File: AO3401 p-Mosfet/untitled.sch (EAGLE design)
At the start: 5 parts

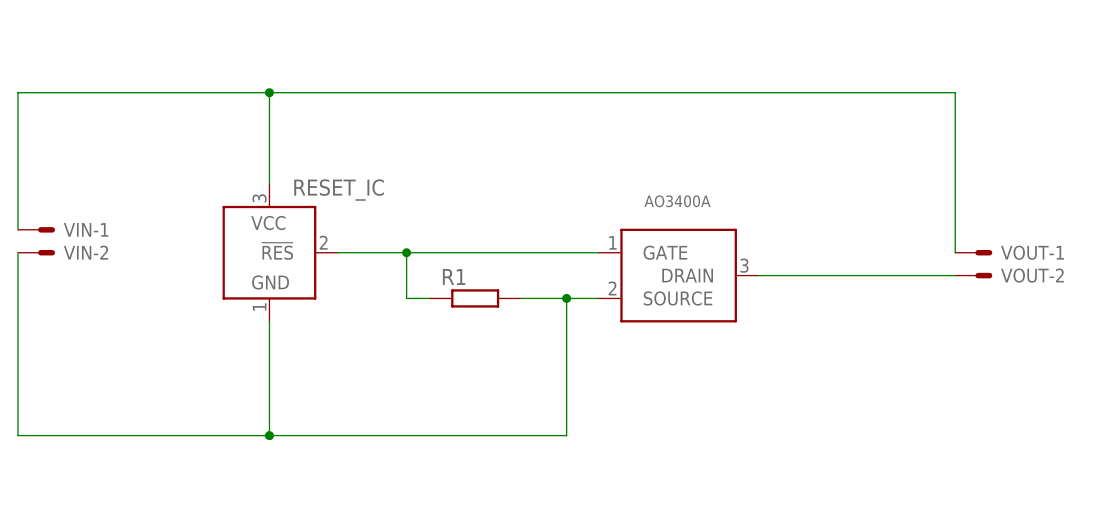
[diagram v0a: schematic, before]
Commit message: new update podlewacz v2
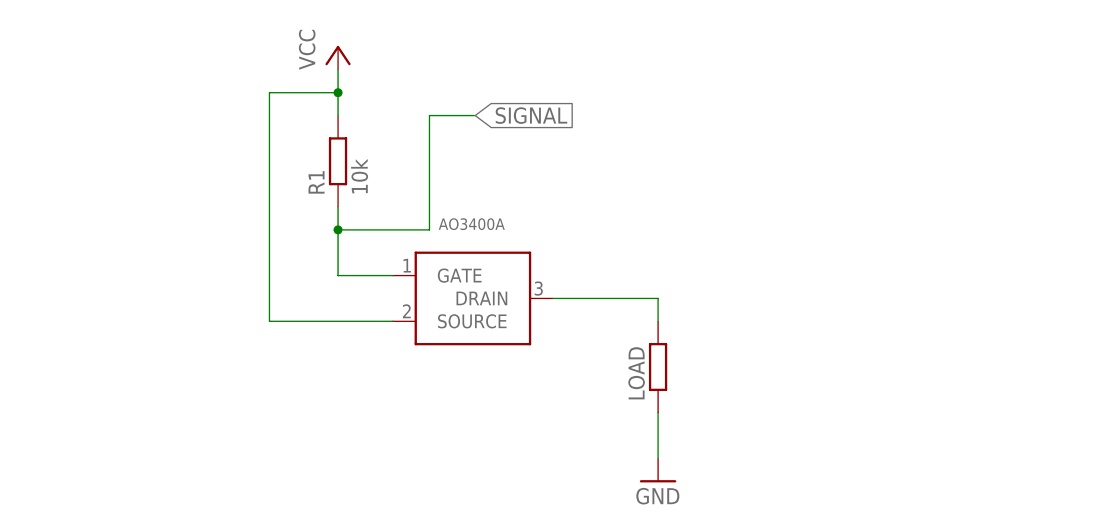
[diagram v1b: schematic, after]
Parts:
- removed MOSFET: AO3400A, smd-footprints:AO3400A
- removed RESET_IC: (no value), telcom:TCM809
- removed VIN, VOUT: 22-23-2021, con-molex:22-23-2021
- added AO3401_P-MOSFET: AO3401_P-MOSFET, smd-footprints:AO3400A
- added LOAD: (no value), resistor:R-EU_0204/2V
- R1: value (none) -> 10k; device resistor:R-EU_R1206 -> resistor:R-EU_0204/2V
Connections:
- removed net N$1: MOSFET.DRAIN, VOUT-2.S
- removed net N$3: MOSFET.GATE, R1.1, RESET_IC.!RES
- new net N$2: AO3401_P-MOSFET.DRAIN, LOAD.2
- new net SIGNAL: AO3401_P-MOSFET.GATE, R1.1
- net GND: now also LOAD.1; no longer MOSFET.SOURCE, R1.2, RESET_IC.GND, VIN-2.S
- net VCC: now also AO3401_P-MOSFET.SOURCE, R1.2; no longer RESET_IC.VCC, VIN-1.S, VOUT-1.S
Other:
- moved on the sheet: R1
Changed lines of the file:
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@@
 </classes>
 <parts>
-<part name="MOSFET" library="smd-footprints" deviceset="AO3400A" device=""/>
-<part name="RESET_IC" library="telcom" deviceset="TCM809" device=""/>
-<part name="VIN" library="con-molex" deviceset="22-23-2021" device="" value=""/>
-<part name="VOUT" library="con-molex" deviceset="22-23-2021" device="" value=""/>
-<part name="R1" library="resistor" deviceset="R-EU_" device="R1206"/>
+<part name="AO3401_P-MOSFET" library="smd-footprints" deviceset="AO3400A" device="" value="AO3401_P-MOSFET"/>
+<part name="GND1" library="supply1" deviceset="GND" device=""/>
+<part name="P+1" library="supply1" deviceset="VCC" device=""/>
+<part name="R1" library="resistor" deviceset="R-EU_" device="0204/2V" value="10k"/>
+<part name="LOAD" library="resistor" deviceset="R-EU_" device="0204/2V"/>
 </parts>
 <sheets>
@@
 </plain>
 <instances>
-<instance part="MOSFET" gate="AO3400A" x="50.8" y="60.96"/>
-<instance part="RESET_IC" gate="G$1" x="5.08" y="63.5"/>
-<instance part="VIN" gate="-1" x="-20.32" y="66.04"/>
-<instance part="VIN" gate="-2" x="-20.32" y="63.5"/>
-<instance part="VOUT" gate="-1" x="83.82" y="63.5"/>
-<instance part="VOUT" gate="-2" x="83.82" y="60.96"/>
-<instance part="R1" gate="G$1" x="27.94" y="58.42"/>
+<instance part="AO3401_P-MOSFET" gate="AO3400A" x="27.94" y="58.42"/>
+<instance part="GND1" gate="1" x="48.26" y="38.1"/>
+<instance part="P+1" gate="VCC" x="12.7" y="86.36"/>
+<instance part="R1" gate="G$1" x="12.7" y="73.66" rot="R90"/>
+<instance part="LOAD" gate="G$1" x="48.26" y="50.8" rot="R90"/>
 </instances>
 <busses>
@@
 <net name="VCC" class="0">
 <segment>
-<wire x1="-22.86" y1="66.04" x2="-22.86" y2="81.28" width="0.1524" layer="91"/>
-<wire x1="-22.86" y1="81.28" x2="5.08" y2="81.28" width="0.1524" layer="91"/>
-<wire x1="5.08" y1="81.28" x2="81.28" y2="81.28" width="0.1524" layer="91"/>
-<wire x1="81.28" y1="81.28" x2="81.28" y2="63.5" width="0.1524" layer="91"/>
-<pinref part="VIN" gate="-1" pin="S"/>
-<pinref part="VOUT" gate="-1" pin="S"/>
-<pinref part="RESET_IC" gate="G$1" pin="VCC"/>
-<wire x1="5.08" y1="71.12" x2="5.08" y2="81.28" width="0.1524" layer="91"/>
-<junction x="5.08" y="81.28"/>
+<pinref part="P+1" gate="VCC" pin="VCC"/>
+<pinref part="R1" gate="G$1" pin="2"/>
+<wire x1="12.7" y1="83.82" x2="12.7" y2="81.28" width="0.1524" layer="91"/>
+<wire x1="12.7" y1="81.28" x2="12.7" y2="78.74" width="0.1524" layer="91"/>
+<wire x1="18.796" y1="55.88" x2="5.08" y2="55.88" width="0.1524" layer="91"/>
+<wire x1="5.08" y1="55.88" x2="5.08" y2="81.28" width="0.1524" layer="91"/>
+<wire x1="5.08" y1="81.28" x2="12.7" y2="81.28" width="0.1524" layer="91"/>
+<junction x="12.7" y="81.28"/>
+<pinref part="AO3401_P-MOSFET" gate="AO3400A" pin="SOURCE"/>
 </segment>
 </net>
-<net name="N$3" class="0">
+<net name="SIGNAL" class="0">
 <segment>
-<pinref part="RESET_IC" gate="G$1" pin="!RES"/>
-<wire x1="12.7" y1="63.5" x2="20.32" y2="63.5" width="0.1524" layer="91"/>
-<pinref part="MOSFET" gate="AO3400A" pin="GATE"/>
 <pinref part="R1" gate="G$1" pin="1"/>
-<wire x1="20.32" y1="63.5" x2="41.656" y2="63.5" width="0.1524" layer="91"/>
-<wire x1="22.86" y1="58.42" x2="20.32" y2="58.42" width="0.1524" layer="91"/>
-<wire x1="20.32" y1="58.42" x2="20.32" y2="63.5" width="0.1524" layer="91"/>
-<junction x="20.32" y="63.5"/>
+<wire x1="18.796" y1="60.96" x2="12.7" y2="60.96" width="0.1524" layer="91"/>
+<wire x1="12.7" y1="60.96" x2="12.7" y2="66.04" width="0.1524" layer="91"/>
+<pinref part="AO3401_P-MOSFET" gate="AO3400A" pin="GATE"/>
+<wire x1="12.7" y1="66.04" x2="12.7" y2="68.58" width="0.1524" layer="91"/>
+<wire x1="12.7" y1="66.04" x2="22.86" y2="66.04" width="0.1524" layer="91"/>
+<wire x1="22.86" y1="66.04" x2="22.86" y2="78.74" width="0.1524" layer="91"/>
+<junction x="12.7" y="66.04"/>
+<wire x1="22.86" y1="78.74" x2="27.94" y2="78.74" width="0.1524" layer="91"/>
+<label x="27.94" y="78.74" size="1.778" layer="95" xref="yes"/>
+</segment>
+</net>
+<net name="N$2" class="0">
+<segment>
+<pinref part="LOAD" gate="G$1" pin="2"/>
+<wire x1="36.576" y1="58.42" x2="48.26" y2="58.42" width="0.1524" layer="91"/>
+<wire x1="48.26" y1="58.42" x2="48.26" y2="55.88" width="0.1524" layer="91"/>
+<pinref part="AO3401_P-MOSFET" gate="AO3400A" pin="DRAIN"/>
 </segment>
 </net>
 <net name="GND" class="0">
 <segment>
-<pinref part="R1" gate="G$1" pin="2"/>
-<wire x1="33.02" y1="58.42" x2="38.1" y2="58.42" width="0.1524" layer="91"/>
-<pinref part="MOSFET" gate="AO3400A" pin="SOURCE"/>
-<wire x1="38.1" y1="58.42" x2="41.656" y2="58.42" width="0.1524" layer="91"/>
-<wire x1="38.1" y1="58.42" x2="38.1" y2="43.18" width="0.1524" layer="91"/>
-<junction x="38.1" y="58.42"/>
-<pinref part="VIN" gate="-2" pin="S"/>
-<wire x1="-22.86" y1="63.5" x2="-22.86" y2="43.18" width="0.1524" layer="91"/>
-<pinref part="RESET_IC" gate="G$1" pin="GND"/>
-<wire x1="-22.86" y1="43.18" x2="5.08" y2="43.18" width="0.1524" layer="91"/>
-<wire x1="5.08" y1="43.18" x2="5.08" y2="55.88" width="0.1524" layer="91"/>
-<wire x1="38.1" y1="43.18" x2="5.08" y2="43.18" width="0.1524" layer="91"/>
-<junction x="5.08" y="43.18"/>
+<pinref part="LOAD" gate="G$1" pin="1"/>
+<pinref part="GND1" gate="1" pin="GND"/>
+<wire x1="48.26" y1="45.72" x2="48.26" y2="40.64" width="0.1524" layer="91"/>
 </segment>
 </net>
-<net name="N$1" class="0">
-<segment>
-<pinref part="VOUT" gate="-2" pin="S"/>
-<pinref part="MOSFET" gate="AO3400A" pin="DRAIN"/>
-<wire x1="59.436" y1="60.96" x2="81.28" y2="60.96" width="0.1524" layer="91"/>
-</segment>
-</net>
